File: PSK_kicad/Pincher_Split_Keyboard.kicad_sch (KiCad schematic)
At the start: 20 parts, among them U1 RP2040_Zero, U2 TRRS

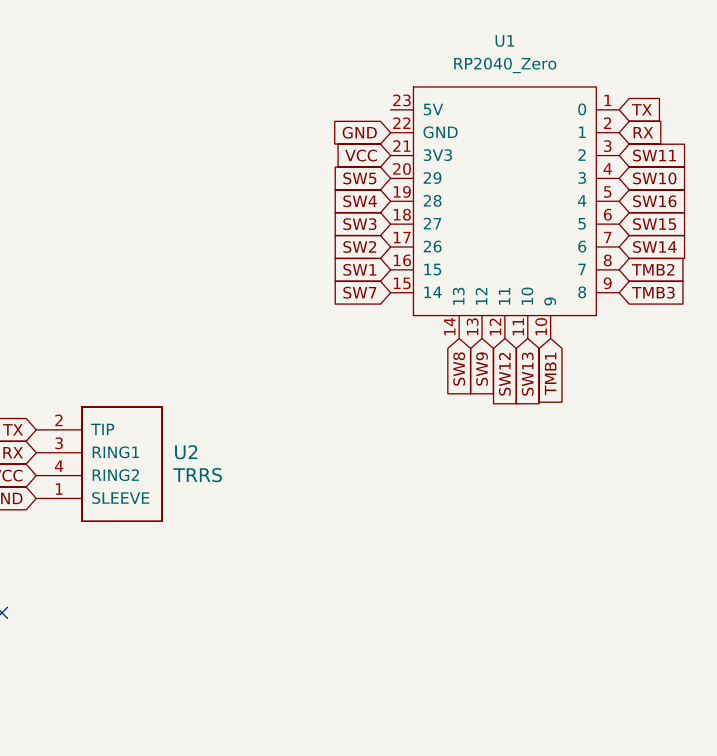
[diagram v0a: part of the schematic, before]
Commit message: fixed rx tx
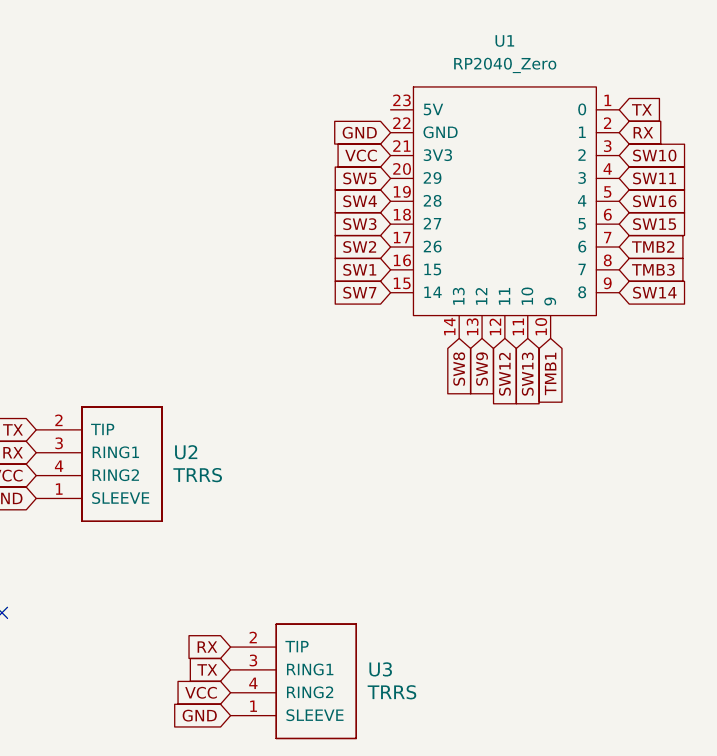
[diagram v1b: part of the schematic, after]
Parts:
- added U3: TRRS, Footprints:Jack_3.5mm_PJ320D_Horizontal, symbol Symbols:Placeholder_TRRS
- U2: footprint Footprints:TRRS_PJ-320A -> Footprints:Jack_3.5mm_PJ320D_Horizontal
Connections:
- net GND: now also U3.1 (SLEEVE)
- net RX: now also U3.2 (TIP)
- net SW10: now also U1.3 (2); no longer U1.4 (3)
- net SW11: now also U1.4 (3); no longer U1.3 (2)
- net SW14: now also U1.9 (8); no longer U1.7 (6)
- net TMB2: now also U1.7 (6); no longer U1.8 (7)
- net TMB3: now also U1.8 (7); no longer U1.9 (8)
- net TX: now also U3.3 (RING1)
- net VCC: now also U3.4 (RING2)
